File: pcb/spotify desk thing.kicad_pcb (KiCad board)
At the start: 2 copper layers, 113 x 50 mm, 46 parts, among them J1 USB_C_Receptacle_USB2.0_16P, J2 AudioJack3_Ground, J3 DFR0669, U1 PCM5242RHBR, U2 TPA6132A2RTER, U3 EC11E18244A5, U4 ESP32-S3-WROOM-1-N4, U5 USBLC6-2SC6

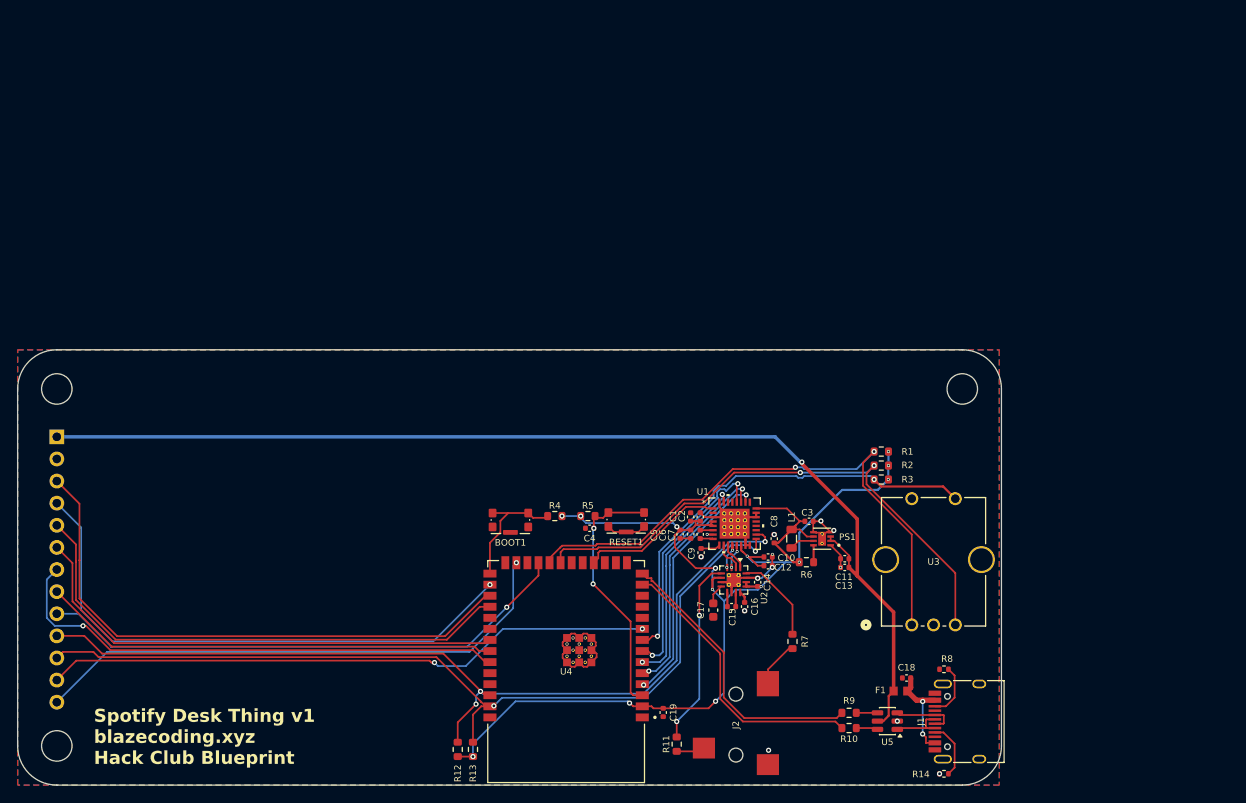
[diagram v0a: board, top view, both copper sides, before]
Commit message: updated pcb with review changes
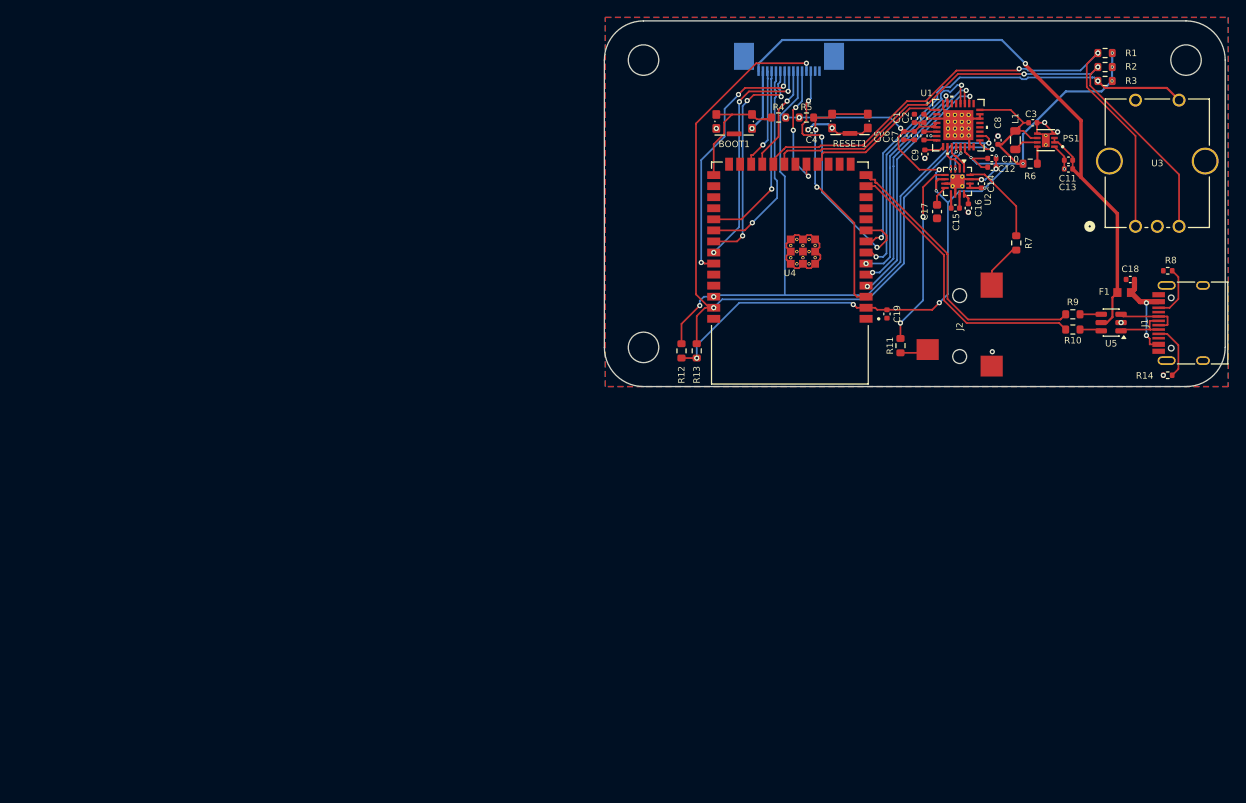
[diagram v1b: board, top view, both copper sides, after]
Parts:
- J3: value DFR0669 -> ST7796; footprint Connector_PinHeader_2.54mm:PinHeader_1x13_P2.54mm_Vertical -> Connector_FFC-FPC:TE_1-1734839-5_1x15-1MP_P0.5mm_Horizontal
- U4: value ESP32-S3-WROOM-1-N4 -> ESP32-S3-WROOM-1-N16R8
- moved J3 94.6 mm to (134.1, 92.1), turned to 0 degrees
- moved C10 52.5 mm to (157.4, 103.5)
- moved C12 52.5 mm to (157.4, 104.5)
- moved R2 52.5 mm to (170.4, 93.0)
- moved R3 52.5 mm to (170.4, 94.6)
- moved R6 52.5 mm to (161.8, 104.1)
- moved BOOT1 52.5 mm to (127.8, 99.3)
- moved R11 52.5 mm to (146.9, 125.0)
- moved R12 52.5 mm to (121.8, 125.6)
- moved R13 52.5 mm to (123.5, 125.6)
- moved C18 52.5 mm to (173.3, 117.4)
- moved R1 52.5 mm to (170.4, 91.4)
- moved U3 52.5 mm to (173.9, 111.3)
- moved C1 52.5 mm to (148.5, 98.9)
- moved C11 52.5 mm to (166.2, 103.7)
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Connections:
- net SCREEN_BL renamed MISO
- net SCREEN_CS renamed MOSI
- net SCREEN_DC renamed LED
- net SCREEN_RES renamed SCK
- J3 pad 11: SDA -> RST
- J3 pad 12: TOUCH_INT -> SDA
- J3 pad 13: SD_CS -> INT
- J3 pad 3: SCREEN_SCLK -> LCD_CS
- J3 pad 4: SCREEN_MOSI -> LCD_RST
- J3 pad 5: SCREEN_MISO -> LCD_RS
- U4 pad 19: unconnected-(U1-IO11-Pad19) -> RST
- U4 pad 24: unconnected-(U1-IO47-Pad24) -> LCD_CS
- U4 pad 28: SCREEN_MOSI -> unconnected-(U4-IO35-Pad28)
- U4 pad 29: SCREEN_SCLK -> unconnected-(U4-IO36-Pad29)
- U4 pad 30: SCREEN_MISO -> unconnected-(U4-IO37-Pad30)
- U4 pad 31: unconnected-(U1-IO38-Pad31) -> LCD_RST
- U4 pad 32: unconnected-(U1-IO39-Pad32) -> LCD_RS
- U4 pad 9: TOUCH_INT -> INT
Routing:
- net TOUCH_INT: track 70.2 -> 0.00 mm, vias 2 -> 0
- net SCREEN_SCLK: track 65.4 -> 0.00 mm
- net SCREEN_MOSI: track 64.6 -> 0.00 mm, vias 1 -> 0
- net SD_CS: track 62.3 -> 0.00 mm, vias 1 -> 0
- net SCREEN_MISO: track 60.5 -> 0.00 mm
- net 5v: track 128.1 -> 75.1 mm
- net MISO: track 61.8 -> 12.2 mm
- net MOSI: track 57.0 -> 26.8 mm, vias 0 -> 3
- net INT: track 0.00 -> 29.8 mm, vias 0 -> 3
- net SCK: track 59.0 -> 29.9 mm, vias 1 -> 3
- net SCL: track 105.6 -> 79.4 mm
- net LED: track 52.6 -> 27.0 mm, vias 0 -> 3
- net LCD_RS: track 0.00 -> 23.7 mm, vias 0 -> 1
- net LCD_RST: track 0.00 -> 21.7 mm, vias 0 -> 1
- net RST: track 0.00 -> 14.7 mm, vias 0 -> 3
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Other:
- board size 113 x 50 mm -> 71.3 x 42 mm
